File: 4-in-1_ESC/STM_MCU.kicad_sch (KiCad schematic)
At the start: 7 parts, among them U12 STM32G071GBU6

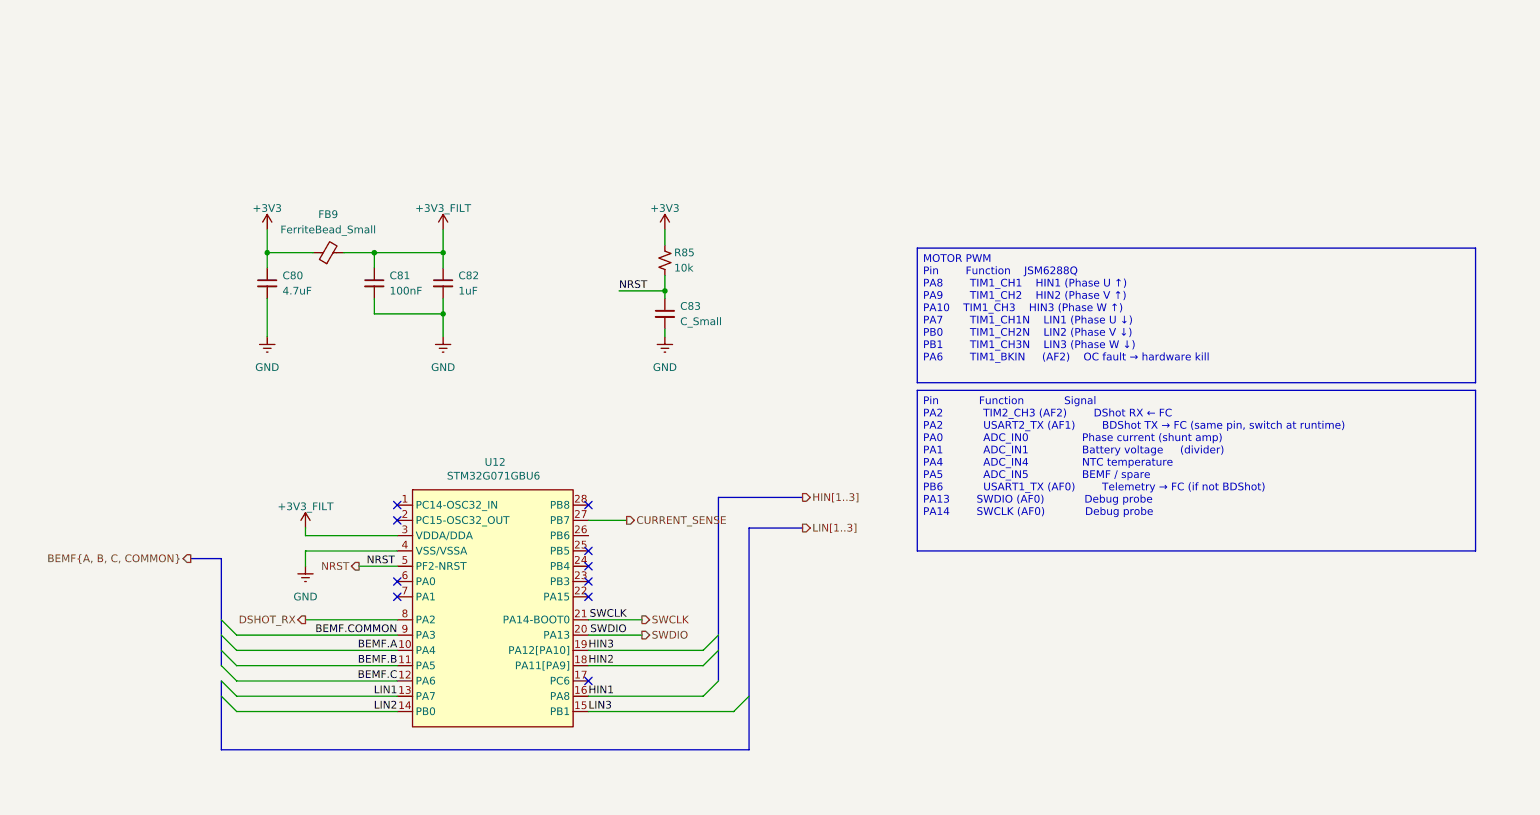
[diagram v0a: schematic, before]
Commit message: Schematic First Pass
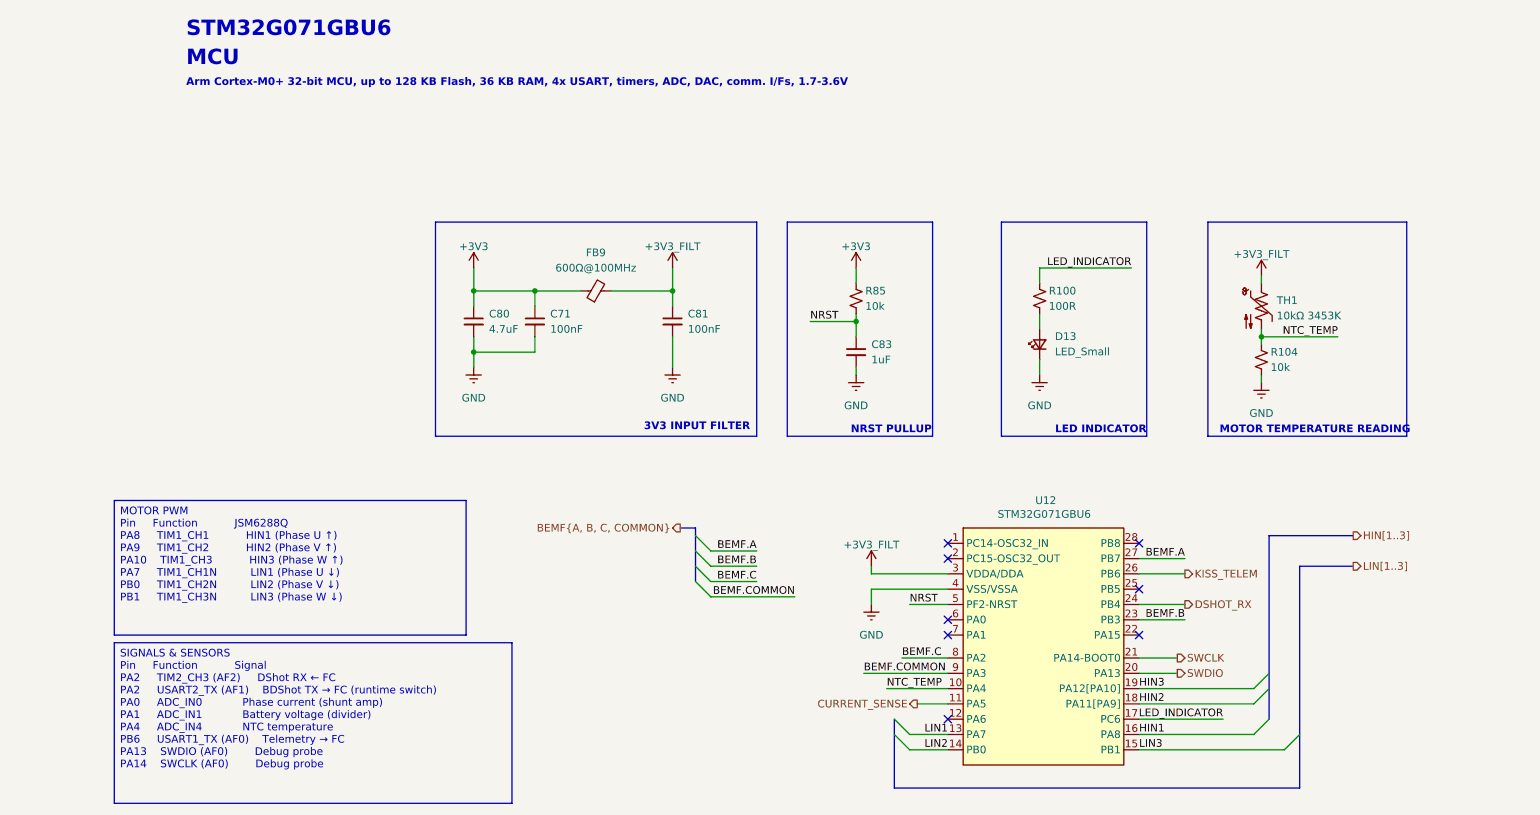
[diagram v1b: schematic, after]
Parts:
- removed C82: 1uF, Capacitor_SMD:C_0402_1005Metric, symbol Device:C_Small
- added C71: 100nF, Capacitor_SMD:C_0402_1005Metric, symbol Device:C_Small
- added D13: LED_Small, symbol Device:LED_Small
- added R100: 100R, Resistor_SMD:R_0402_1005Metric, symbol Device:R_Small_US
- added R104: 10k, Resistor_SMD:R_0402_1005Metric, symbol Device:R_Small_US
- added TH1: 10kΩ 3453K, symbol Device:Thermistor_NTC_US
- C83: value C_Small -> 1uF
- FB9: value FerriteBead_Small -> 600Ω@100MHz; LCSC_Part_Number (none) -> C160977
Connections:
- net +3V3: now also C71.1
- net +3V3_FILT: now also TH1.1
- net BEMF.A: now also U12.27 (PB7); no longer U12.10 (PA4)
- net BEMF.B: now also U12.23 (PB3); no longer U12.11 (PA5)
- net BEMF.C: now also U12.8 (PA2); no longer U12.12 (PA6)
- net CURRENT_SENSE: now also U12.11 (PA5); no longer U12.27 (PB7)
- net DSHOT_RX: now also U12.24 (PB4); no longer U12.8 (PA2)
- net GND: now also C71.2, D13.1 (K), R104.2
- net LED_INDICATOR: now reaches U12.17 (PC6)
- net LED_INDICATOR: now also R100.1
- net KISS_TELEM: now reaches U12.26 (PB6)
- new net: D13.2 (A), R100.2
- new net NTC_TEMP: R104.1, TH1.2, U12.10 (PA4)
- no-connect marks 10 -> 8
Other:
- note added: "3V3 INPUT FILTER"
- note added: "Arm Cortex-M0+ 32-bit MCU, up to 128 KB Flash, 36 KB RAM, 4x USART, timers, ADC, DAC, comm. I/Fs, 1.7-3.6V"
- note added: "LED INDICATOR"
- note added: "MCU"
- note added: "MOTOR TEMPERATURE READING"
- note added: "NRST PULLUP"
- note added: "STM32G071GBU6"
- moved on the sheet: C81, C83, FB9, R85, U12
